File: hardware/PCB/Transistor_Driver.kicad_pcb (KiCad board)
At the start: 2 copper layers, 50 x 50 mm, 11 parts, among them J1 Conn_5V, J2 Conn_GND, J3 Power_Output, K1 G5LE-1, Q1 BC547

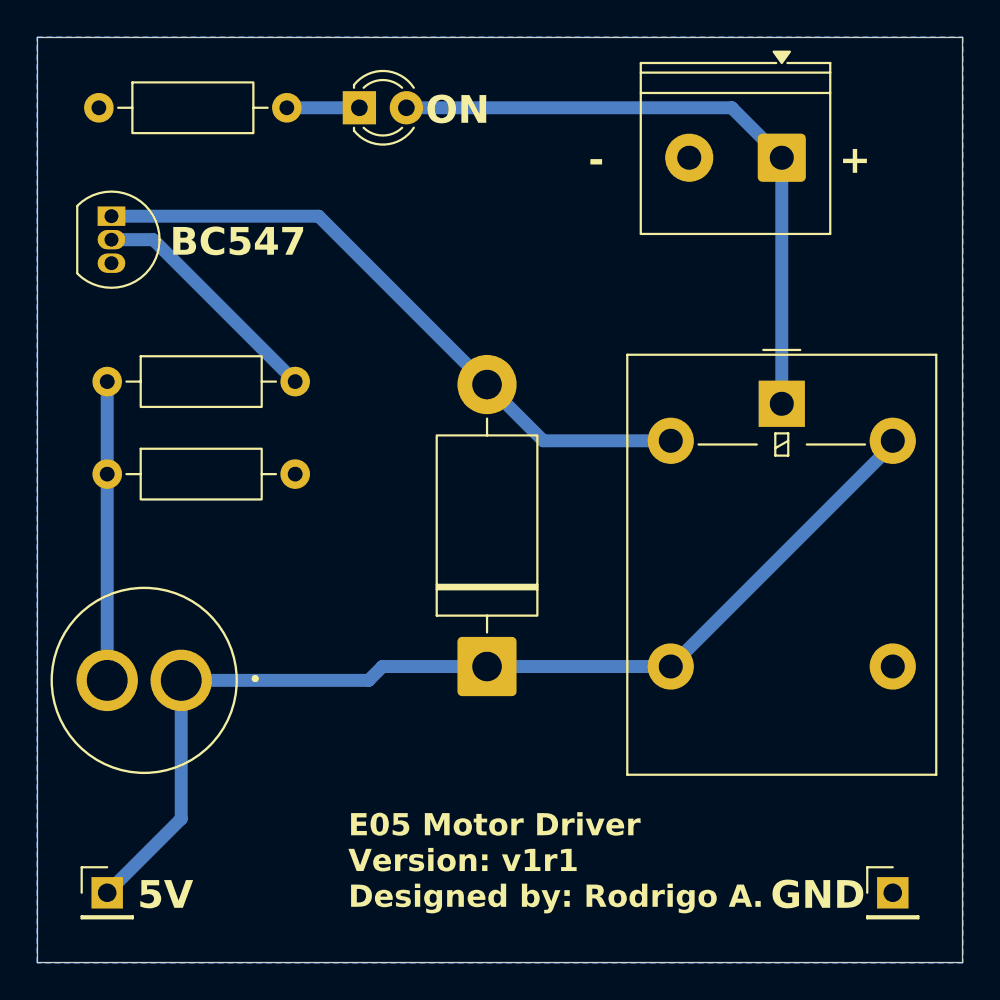
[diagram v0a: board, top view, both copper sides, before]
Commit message: feat(hardware): release v1r2
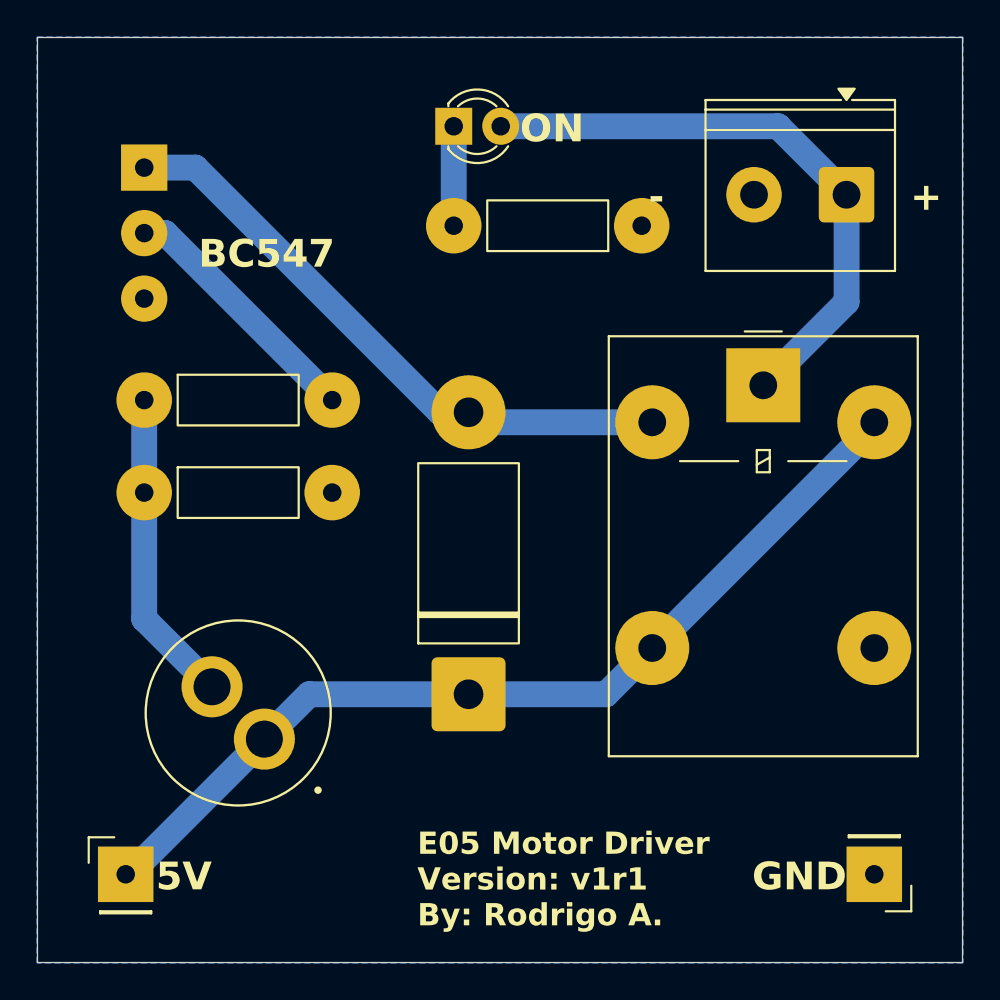
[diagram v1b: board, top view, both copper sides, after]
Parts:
- D1: footprint Diode_THT:D_DO-201AD_P15.24mm_Horizontal -> Transistor_Driver-Footprints:D_DO-201AD_P15.24mm_Horizontal
- D2: footprint LED_THT:LED_D3.0mm -> Transistor_Driver-Footprints:LED_D3.0mm_Clear
- J1, J2: footprint Connector_PinHeader_2.54mm:PinHeader_1x01_P2.54mm_Vertical -> Transistor_Driver-Footprints:PinHeader_1x01_P2.54mm_Vertical
- J3: footprint TerminalBlock_Phoenix:TerminalBlock_Phoenix_PT-1,5-2-5.0-H_1x02_P5.00mm_Horizontal -> Transistor_Driver-Footprints:TerminalBlock_Phoenix_PT-1,5-2-5.0-H_1x02_P5.00mm_Horizontal
- K1: footprint Relay_THT:Relay_SPDT_Omron-G5LE-1 -> Transistor_Driver-Footprints:Relay_SPDT_Omron-G5LE-1
- Q1: footprint Package_TO_SOT_THT:TO-92_Inline -> Transistor_Driver-Footprints:TO-92_Inline_Wide
- R1, R2, R3: footprint Resistor_THT:R_Axial_DIN0207_L6.3mm_D2.5mm_P10.16mm_Horizontal -> Transistor_Driver-Footprints:R_Axial_DIN0207_L6.3mm_D2.5mm_P10.16mm_Horizontal
- S1: footprint PS1024ALRED:SW_PS1024ALRED -> Transistor_Driver-Footprints:SW_PS1024ALRED
- moved R3 30.0 mm to (207.9, 62.2), turned to 180 degrees
- moved S1 5.38 mm to (186.1, 88.5), turned to 135 degrees
- moved D2 5.20 mm to (197.7, 56.8)
- moved J3 4.03 mm to (218.9, 60.5)
- moved Q1 2.40 mm to (181.0, 60.0)
- moved R1 2.24 mm to (181.0, 76.6)
- moved R2 2.24 mm to (181.0, 71.6)
- moved D1 1.80 mm to (198.5, 87.5)
- moved J1 1.41 mm to (180.0, 97.2)
- moved J2 1.41 mm to (220.4, 97.2), turned to 180 degrees
- moved K1 1.41 mm to (214.4, 70.8)
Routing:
- net +5V: track 57.1 -> 50.7 mm
- net Net-(D2-A): track 34.7 -> 32.4 mm
- net Net-(D1-A): track 35.3 -> 33.2 mm
- net Net-(D2-K): track 3.92 -> 5.38 mm
- net Net-(Q1-B): track 13.1 -> 14.3 mm
- net Net-(R1-Pad1): track 16.2 -> 17.0 mm
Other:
- board text added: "E05 Motor Driver Version: v1r1 By: Rodrigo A."
- board text removed: "E05 Motor Driver Version: v1r1 Designed by: Rodrigo A."
